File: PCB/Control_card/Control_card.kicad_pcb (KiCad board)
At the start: 2 copper layers, 71.4 x 45.4 mm, 46 parts, among them IC1 TLSR8253F512ET48, J1 Conn_02x04_Counter_Clockwise, J2 Conn_01x01_Pin, J3 Conn_01x01_Pin, J4 Conn_01x01_Pin, J5 Conn_01x01_Pin, Y1 Crystal_GND24

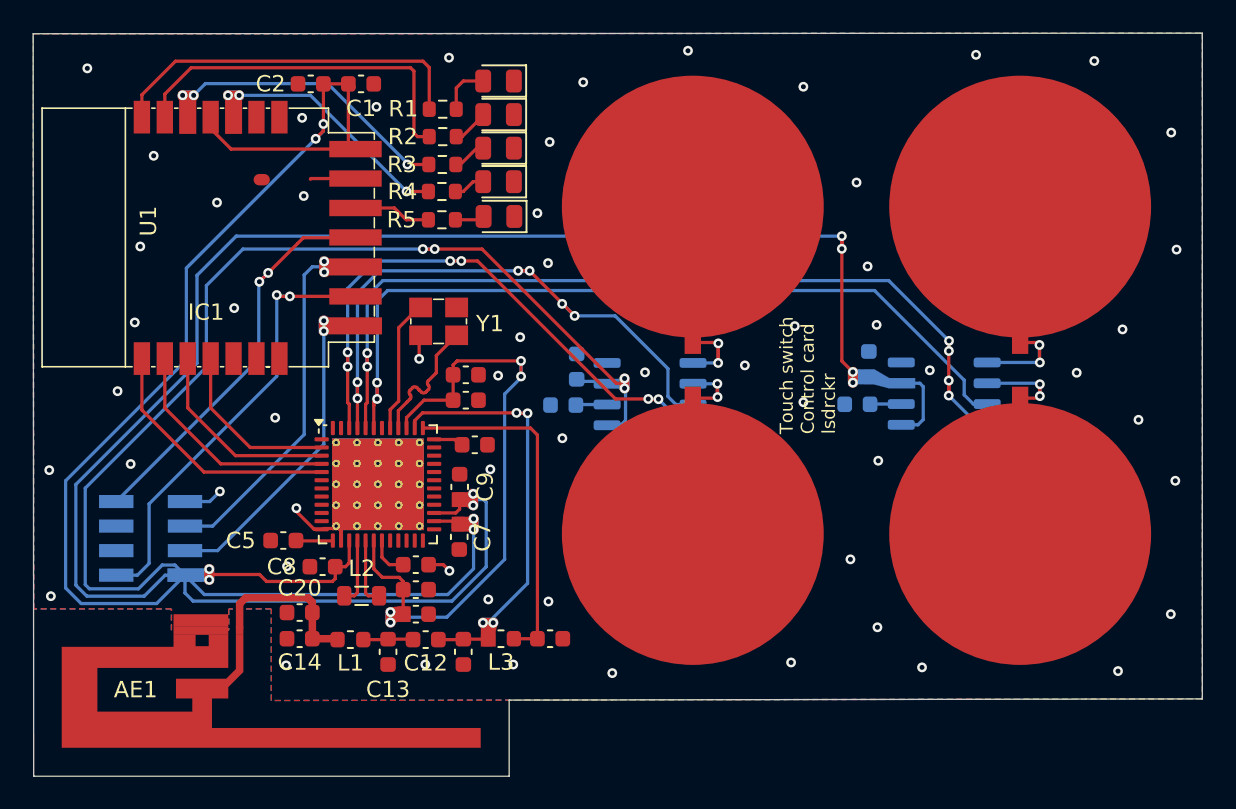
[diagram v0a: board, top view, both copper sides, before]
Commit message: Rota IC contrôle
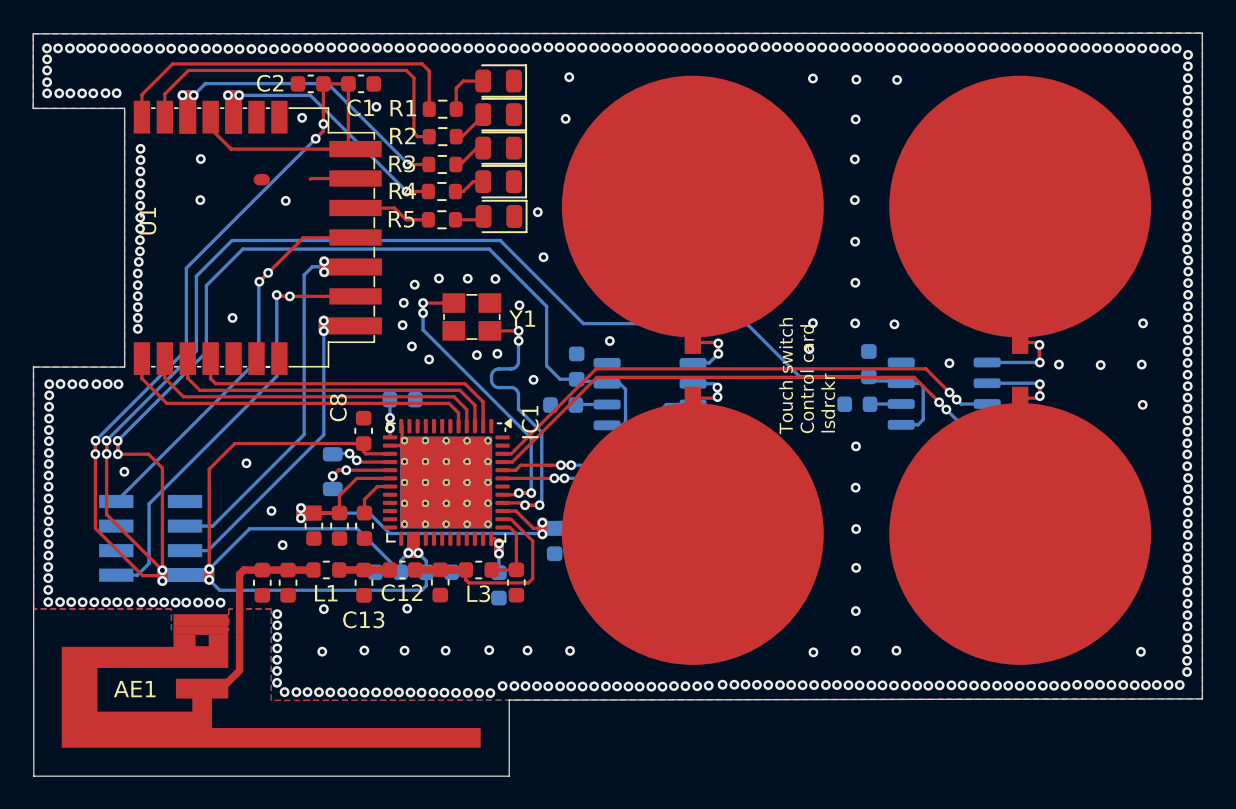
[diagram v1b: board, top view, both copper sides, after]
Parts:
- C15, C16, C17, C5, C7, C9, L2: moved to B.Cu
- moved C15 11.5 mm to (157.4, 77.0), turned to -90 degrees
- moved C5 11.3 mm to (148.1, 68.4), turned to 0 degrees
- moved C16 11.1 mm to (158.9, 77.0), turned to -90 degrees
- moved C17 8.72 mm to (154.0, 79.7), turned to -90 degrees
- moved C8 8.67 mm to (145.7, 70.3), turned to 90 degrees
- moved C6 8.24 mm to (142.7, 76.1), turned to -90 degrees
- moved L2 7.79 mm to (143.8, 72.8), turned to 90 degrees
- moved C4 6.08 mm to (144.2, 76.1), turned to -90 degrees
- moved C9 5.37 mm to (150.3, 78.9), turned to 0 degrees
- moved C7 4.86 mm to (147.2, 78.9), turned to 180 degrees
- moved L1 4.50 mm to (143.4, 78.8)
- moved C12 4.48 mm to (148.1, 78.8)
- moved C13 4.47 mm to (145.7, 79.6)
- moved C11 4.47 mm to (150.4, 79.6)
- moved L3 4.41 mm to (152.7, 78.8)
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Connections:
- IC1 pad 43: OutSw1 -> OutSw4
- IC1 pad 44: OutSw2 -> OutSw3
- IC1 pad 45: OutSw3 -> OutSw2
- IC1 pad 46: OutSw4 -> OutSw1
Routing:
- net GND: track 74.5 -> 5.82 mm, vias 59 -> 372
- net 3.3V: track 275.0 -> 240.9 mm, vias 16 -> 14
- net OutSw3: track 38.2 -> 13.9 mm, vias 6 -> 2
- net OutSw4: track 37.6 -> 13.6 mm, vias 6 -> 2
- net OutSw2: track 57.0 -> 33.6 mm, vias 6 -> 2
- net OutSw1: track 49.8 -> 33.3 mm
- net Net-(IC1-VANT): track 21.1 -> 4.72 mm
- net ANT: track 25.1 -> 12.7 mm, vias 4 -> 0
- net VVD1V2: track 38.1 -> 26.8 mm
- net XC2: track 8.20 -> 19.4 mm, vias 0 -> 4
- net XC1: track 8.13 -> 19.3 mm, vias 0 -> 4
- net In4: track 10.8 -> 19.9 mm
- net In3: track 12.4 -> 20.7 mm
- net In2: track 14.0 -> 21.5 mm
- net In1: track 15.7 -> 22.2 mm
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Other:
- outline, holes or cut-outs redrawn
